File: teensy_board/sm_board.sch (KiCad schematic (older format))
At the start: 53 parts, among them IC1 DRV8833RTYT, J1 Conn_01x06, J10 Conn_01x03, J11 CONN_01X02, J12 CONN_02X04, J13 Conn_01x02, J14 Conn_01x02, J2 Conn_01x06, J3 Conn_01x06, J4 Conn_01x03, J5 Conn_01x03, J6 Conn_01x03, J7 Conn_01x03, J8 Conn_01x03, J9 Conn_01x03, U1 Teensy3.6, U3 tps82130

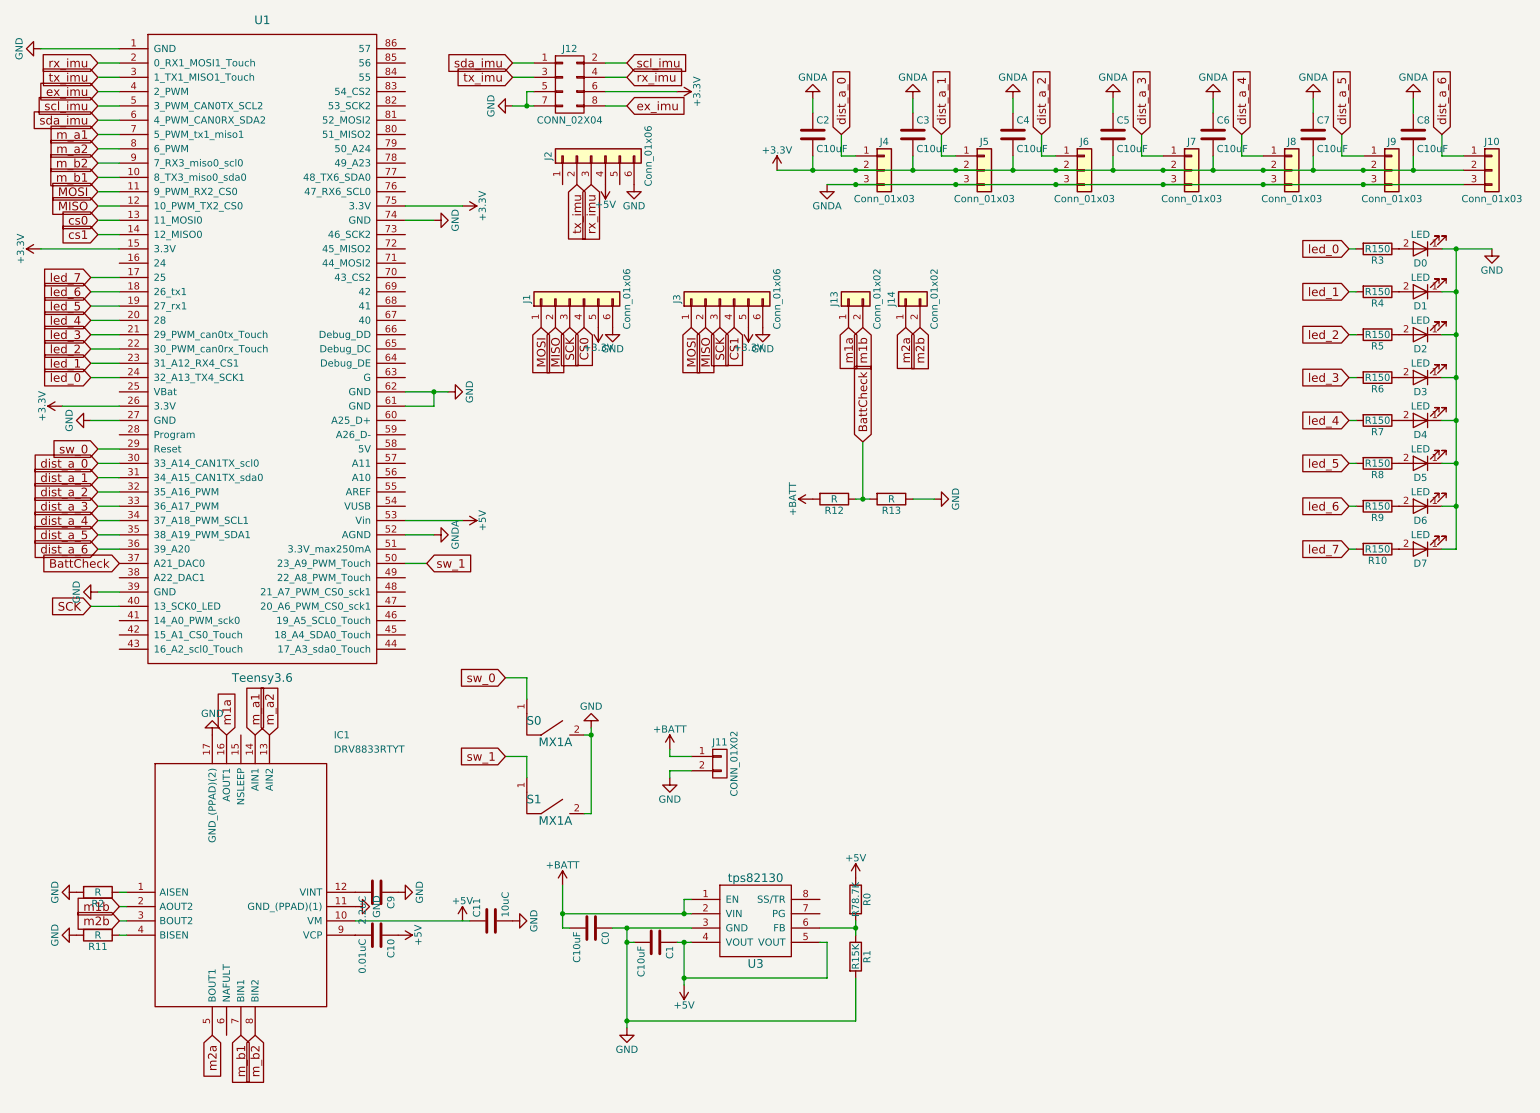
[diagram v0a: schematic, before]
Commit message: After review meeting
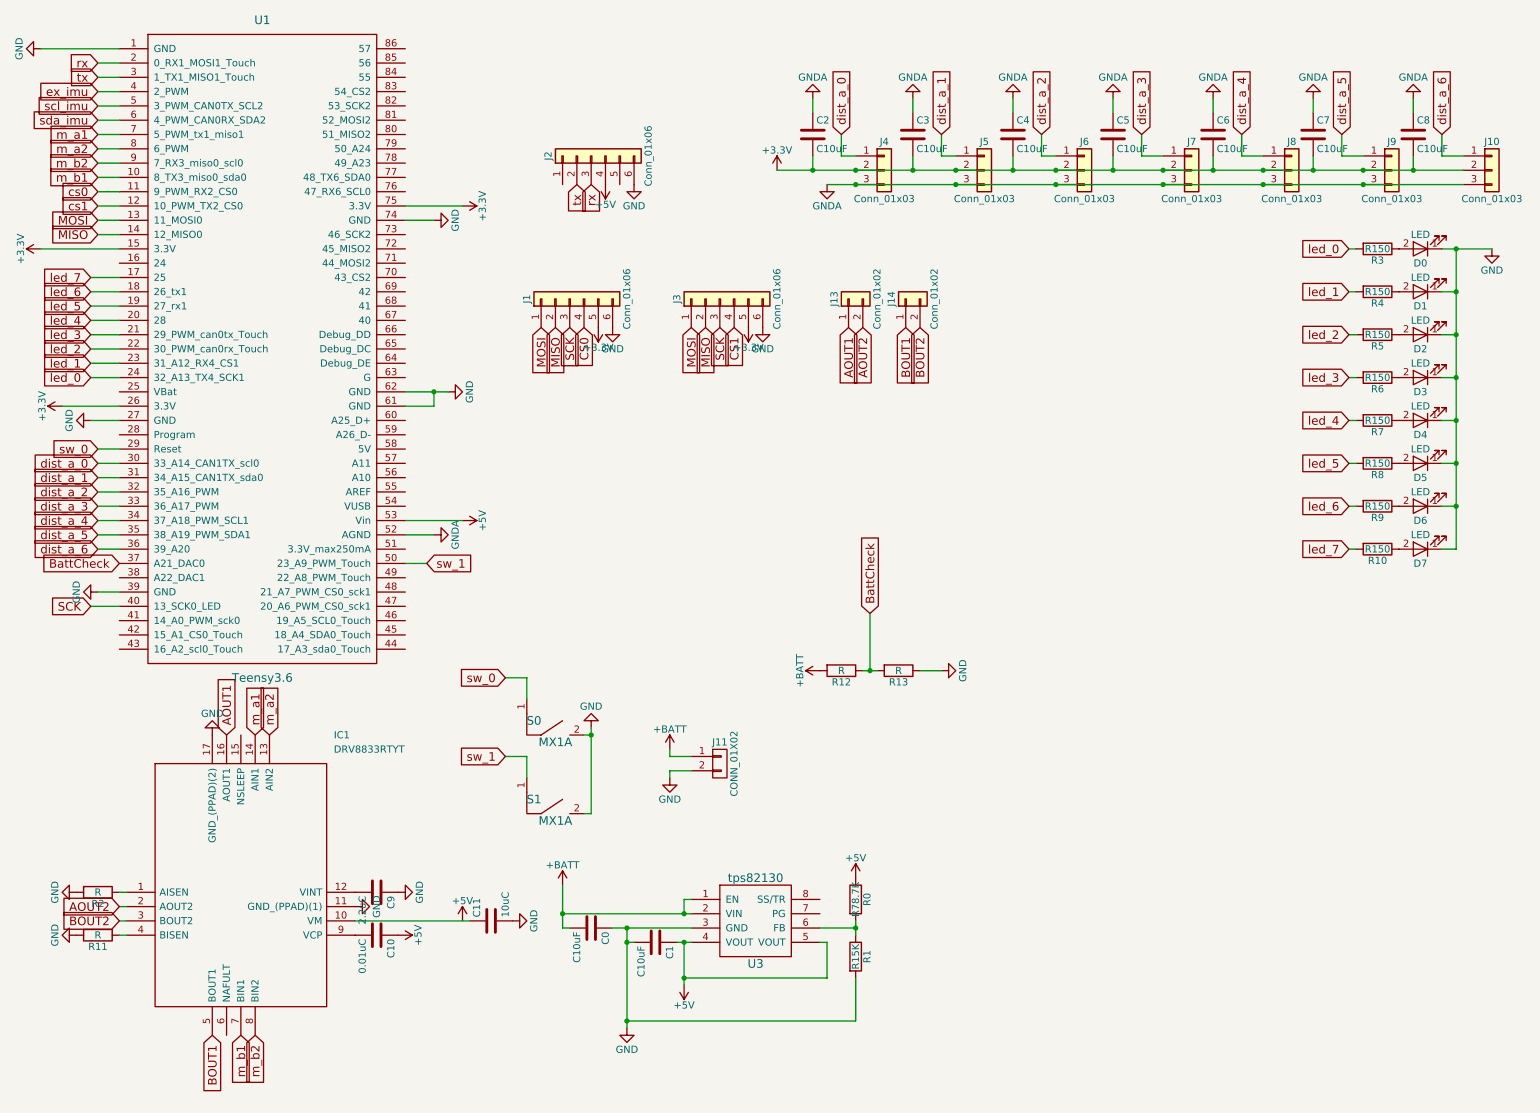
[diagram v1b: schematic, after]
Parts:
- removed J12: CONN_02X04, Pin_Headers:Pin_Header_Straight_2x04_Pitch2.54mm, symbol CONN_02X04
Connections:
- net MISO: now also U1.14 (12_MISO0); no longer U1.12 (10_PWM_TX2_CS0)
- net MOSI: now also U1.13 (11_MOSI0); no longer U1.11 (9_PWM_RX2_CS0)
- net cs0: now also U1.11 (9_PWM_RX2_CS0); no longer U1.13 (11_MOSI0)
- net cs1: now also U1.12 (10_PWM_TX2_CS0); no longer U1.14 (12_MISO0)
- net m1a renamed AOUT1
- net m1b renamed AOUT2
- net m2a renamed BOUT1
- net m2b renamed BOUT2
- net rx_imu renamed rx
- net tx_imu renamed tx
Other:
- moved on the sheet: R12, R13
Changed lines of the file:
@@
 Wire Wire Line
 	3250 1800 3450 1800
-$Comp
-L CONN_02X04 J12
-U 1 1 58ECF8BE
-P 4400 850
-F 0 "J12" H 4400 1100 50  0000 C CNN
-F 1 "CONN_02X04" H 4400 600 50  0000 C CNN
-F 2 "Pin_Headers:Pin_Header_Straight_2x04_Pitch2.54mm" H 4400 -350 50  0001 C CNN
-F 3 "" H 4400 -350 50  0001 C CNN
-	1    4400 850
-	1    0    0    -1
-$EndComp
-Text GLabel 4000 700  0    60   Input ~ 0
-sda_imu
-Text GLabel 4000 800  0    60   Input ~ 0
-tx_imu
-Text GLabel 4800 700  2    60   Input ~ 0
-scl_imu
-Text GLabel 4800 800  2    60   Input ~ 0
-rx_imu
-Text GLabel 4800 1000 2    60   Input ~ 0
-ex_imu
-Wire Wire Line
-	4000 700  4150 700
-Wire Wire Line
-	4000 800  4150 800
-Wire Wire Line
-	4800 700  4650 700
-Wire Wire Line
-	4650 800  4800 800
-Wire Wire Line
-	4800 1000 4650 1000
-$Comp
-L GND #PWR025
-U 1 1 58ED2351
-P 4000 1000
-F 0 "#PWR025" H 4000 750 50  0001 C CNN
-F 1 "GND" H 4000 850 50  0000 C CNN
-F 2 "" H 4000 1000 50  0001 C CNN
-F 3 "" H 4000 1000 50  0001 C CNN
-	1    4000 1000
-	0    1    1    0
-$EndComp
-Wire Wire Line
-	4000 1000 4150 1000
-Wire Wire Line
-	4150 900  4100 900
-Wire Wire Line
-	4100 900  4100 1000
-Connection ~ 4100 1000
-$Comp
-L +3.3V #PWR026
-U 1 1 58ED3028
-P 5150 900
-F 0 "#PWR026" H 5150 750 50  0001 C CNN
-F 1 "+3.3V" H 5150 1040 50  0000 C CNN
-F 2 "" H 5150 900 50  0001 C CNN
-F 3 "" H 5150 900 50  0001 C CNN
-	1    5150 900
-	0    1    1    0
-$EndComp
-Wire Wire Line
-	4650 900  5150 900
 Text GLabel 1100 800  0    60   Input ~ 0
-tx_imu
+tx
 Text GLabel 1100 700  0    60   Input ~ 0
-rx_imu
+rx
 Wire Wire Line
 	1100 1200 1250 1200
@@
 Wire Wire Line
 	3250 3100 3450 3100
+Text GLabel 1100 1800 0    60   Input ~ 0
+MOSI
+Text GLabel 1100 1900 0    60   Input ~ 0
+MISO
 Text GLabel 1100 1600 0    60   Input ~ 0
-MOSI
+cs0
 Text GLabel 1100 1700 0    60   Input ~ 0
-MISO
-Text GLabel 1100 1800 0    60   Input ~ 0
-cs0
-Text GLabel 1100 1900 0    60   Input ~ 0
 cs1
 Wire Wire Line
@@
 $EndComp
 Text GLabel 2000 5400 1    60   Input ~ 0
-m1a
+AOUT1
 Text GLabel 1250 6600 0    60   Input ~ 0
-m1b
+AOUT2
 Text GLabel 1250 6700 0    60   Input ~ 0
-m2b
+BOUT2
 Text GLabel 1900 7500 3    60   Input ~ 0
-m2a
+BOUT1
 Wire Wire Line
 	2900 6700 3700 6700
@@
 $EndComp
 Text GLabel 4450 1550 3    60   Input ~ 0
-tx_imu
+tx
 Text GLabel 4550 1550 3    60   Input ~ 0
-rx_imu
+rx
 $Comp
 L +5V #PWR034
@@
 $EndComp
 Text GLabel 6350 2550 3    60   Input ~ 0
-m1a
+AOUT1
 Text GLabel 6450 2550 3    60   Input ~ 0
-m1b
+AOUT2
 Text GLabel 6750 2550 3    60   Input ~ 0
-m2a
+BOUT1
 Text GLabel 6850 2550 3    60   Input ~ 0
-m2b
+BOUT2
 $Comp
 L GND #PWR040
@@
 L R R12
 U 1 1 5AAC0D56
-P 6250 3750
-F 0 "R12" V 6330 3750 50  0000 C CNN
-F 1 "R" V 6250 3750 50  0000 C CNN
-F 2 "Resistors_SMD:R_0402" V 6180 3750 50  0001 C CNN
-F 3 "" H 6250 3750 50  0001 C CNN
-	1    6250 3750
+P 6300 4950
+F 0 "R12" V 6380 4950 50  0000 C CNN
+F 1 "R" V 6300 4950 50  0000 C CNN
+F 2 "Resistors_SMD:R_0402" V 6230 4950 50  0001 C CNN
+F 3 "" H 6300 4950 50  0001 C CNN
+	1    6300 4950
 	0    1    1    0
 $EndComp
@@
 L R R13
 U 1 1 5AAC0DE4
-P 6650 3750
-F 0 "R13" V 6730 3750 50  0000 C CNN
-F 1 "R" V 6650 3750 50  0000 C CNN
-F 2 "Resistors_SMD:R_0402" V 6580 3750 50  0001 C CNN
-F 3 "" H 6650 3750 50  0001 C CNN
-	1    6650 3750
-	0    1    1    0
-$EndComp
-Wire Wire Line
-	6400 3750 6500 3750
-Wire Wire Line
-	6450 3350 6450 3750
-Connection ~ 6450 3750
-Wire Wire Line
-	6800 3750 6950 3750
+P 6700 4950
+F 0 "R13" V 6780 4950 50  0000 C CNN
+F 1 "R" V 6700 4950 50  0000 C CNN
+F 2 "Resistors_SMD:R_0402" V 6630 4950 50  0001 C CNN
+F 3 "" H 6700 4950 50  0001 C CNN
+	1    6700 4950
+	0    1    1    0
+$EndComp
+Wire Wire Line
+	6450 4950 6550 4950
+Wire Wire Line
+	6500 4550 6500 4950
+Connection ~ 6500 4950
+Wire Wire Line
+	6850 4950 7000 4950
 $Comp
 L GND #PWR041
 U 1 1 5AAC11C8
-P 6950 3750
-F 0 "#PWR041" H 6950 3500 50  0001 C CNN
-F 1 "GND" H 6950 3600 50  0000 C CNN
-F 2 "" H 6950 3750 50  0001 C CNN
-F 3 "" H 6950 3750 50  0001 C CNN
-	1    6950 3750
+P 7000 4950
+F 0 "#PWR041" H 7000 4700 50  0001 C CNN
+F 1 "GND" H 7000 4800 50  0000 C CNN
+F 2 "" H 7000 4950 50  0001 C CNN
+F 3 "" H 7000 4950 50  0001 C CNN
+	1    7000 4950
 	0    -1   -1   0
 $EndComp
@@
 L +BATT #PWR042
 U 1 1 5AAC127B
-P 6100 3750
-F 0 "#PWR042" H 6100 3600 50  0001 C CNN
-F 1 "+BATT" H 6100 3890 50  0000 C CNN
-F 2 "" H 6100 3750 50  0001 C CNN
-F 3 "" H 6100 3750 50  0001 C CNN
-	1    6100 3750
+P 6150 4950
+F 0 "#PWR042" H 6150 4800 50  0001 C CNN
+F 1 "+BATT" H 6150 5090 50  0000 C CNN
+F 2 "" H 6150 4950 50  0001 C CNN
+F 3 "" H 6150 4950 50  0001 C CNN
+	1    6150 4950
 	0    -1   -1   0
 $EndComp
 Text GLabel 1250 4200 0    60   Input ~ 0
 BattCheck
-Text GLabel 6450 3350 1    60   Input ~ 0
+Text GLabel 6500 4550 1    60   Input ~ 0
 BattCheck
 $Comp
